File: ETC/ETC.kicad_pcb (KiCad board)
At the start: 2 copper layers, 96.5 x 100.5 mm, 36 parts, among them P1 DTM1312PC12PDR008, U1 NUCLEO-F446RE, U2 MCP6004, U3 LM7805_TO220, U4 LM7809_TO220, U5 ISO1050DUB, U6 ISO1050DUB, U7 SN74AHC14N

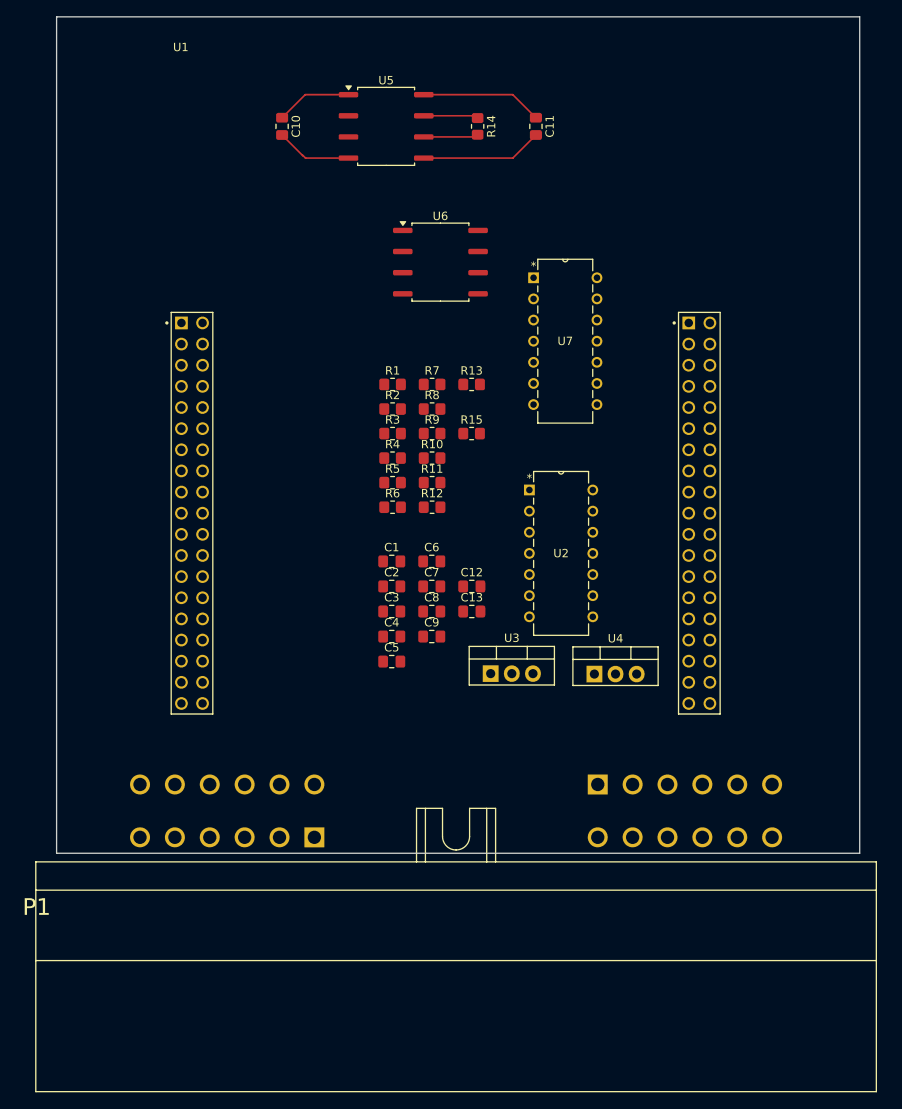
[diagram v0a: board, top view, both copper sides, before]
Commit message: brake light and RTDS
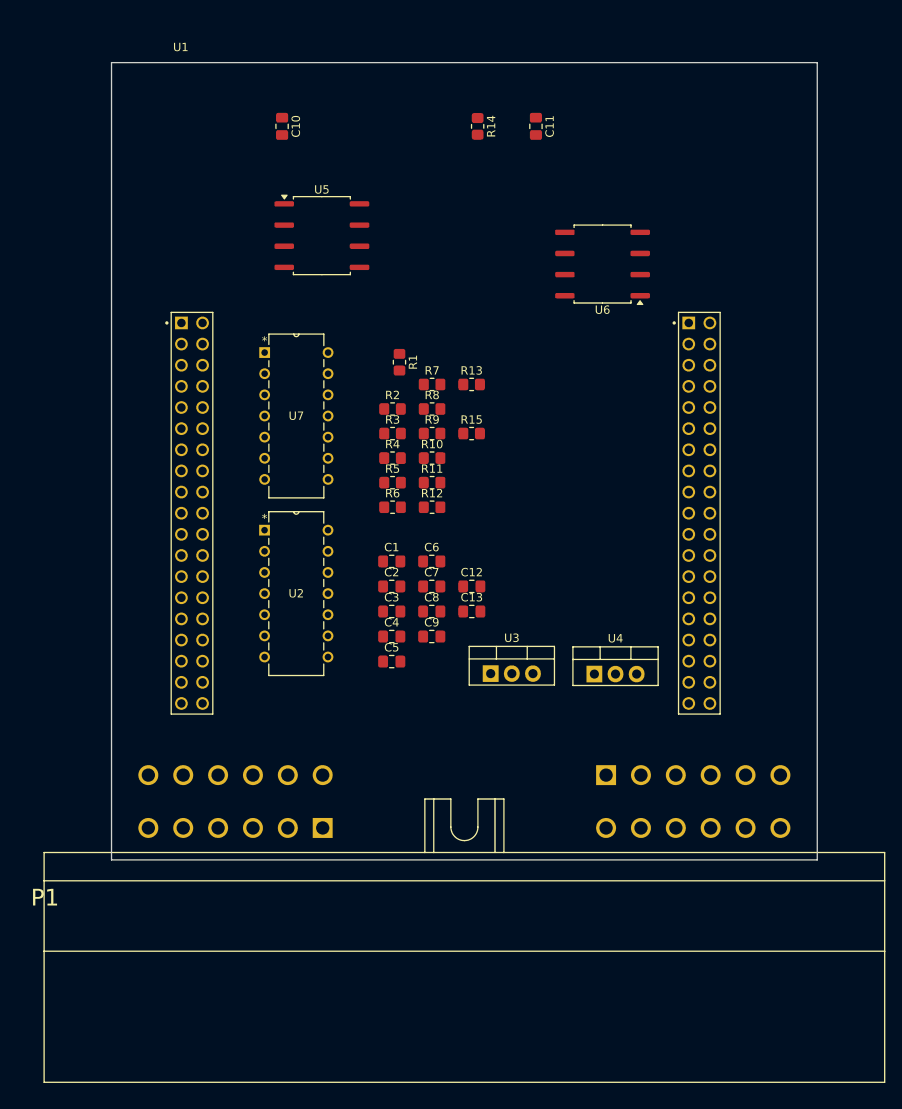
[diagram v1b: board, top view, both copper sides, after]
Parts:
- moved U7 33.5 mm to (183.6, 117.1)
- moved U2 32.2 mm to (183.6, 138.4)
- moved U6 19.5 mm to (216.6, 91.2), turned to 180 degrees
- moved U5 15.2 mm to (182.9, 87.8)
- moved R1 2.80 mm to (192.2, 103.0), turned to -90 degrees
- moved P1 1.51 mm to (200.0, 157.0)
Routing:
- net GND: track 23.7 -> 0.00 mm
- net +5V: track 14.6 -> 0.00 mm
- net +3V3: track 9.12 -> 0.00 mm
- net /L_Motor_CAN: track 6.59 -> 0.38 mm
- net /H_Motor_CAN: track 6.59 -> 0.38 mm
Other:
- board size 96.5 x 100.5 mm -> 84.8 x 95.8 mm
